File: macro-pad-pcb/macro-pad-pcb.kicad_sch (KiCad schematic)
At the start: 46 parts, among them SW1 SW_Push, SW2 RotaryEncoder, U1 PRTR5V0U2X, U2 ATmega32U4-A, Y1 Crystal_GND24_Small

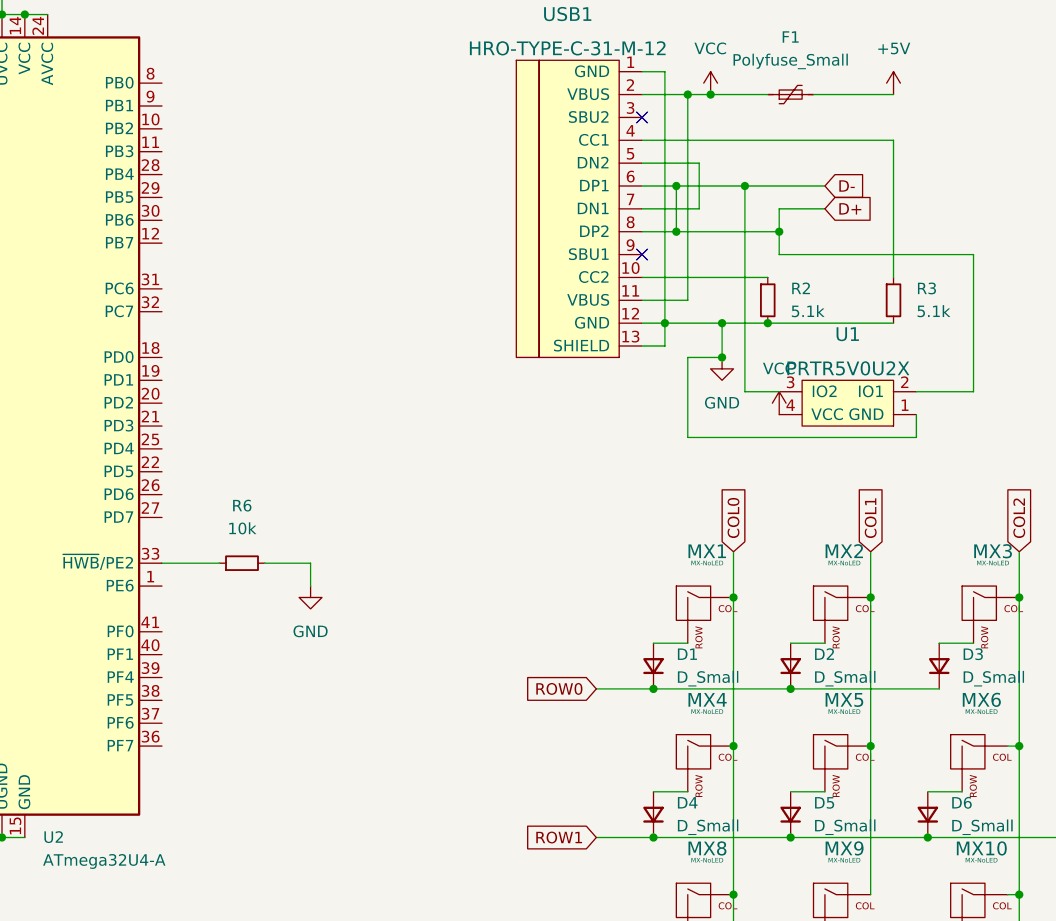
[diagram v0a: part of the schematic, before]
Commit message: Finished PCB
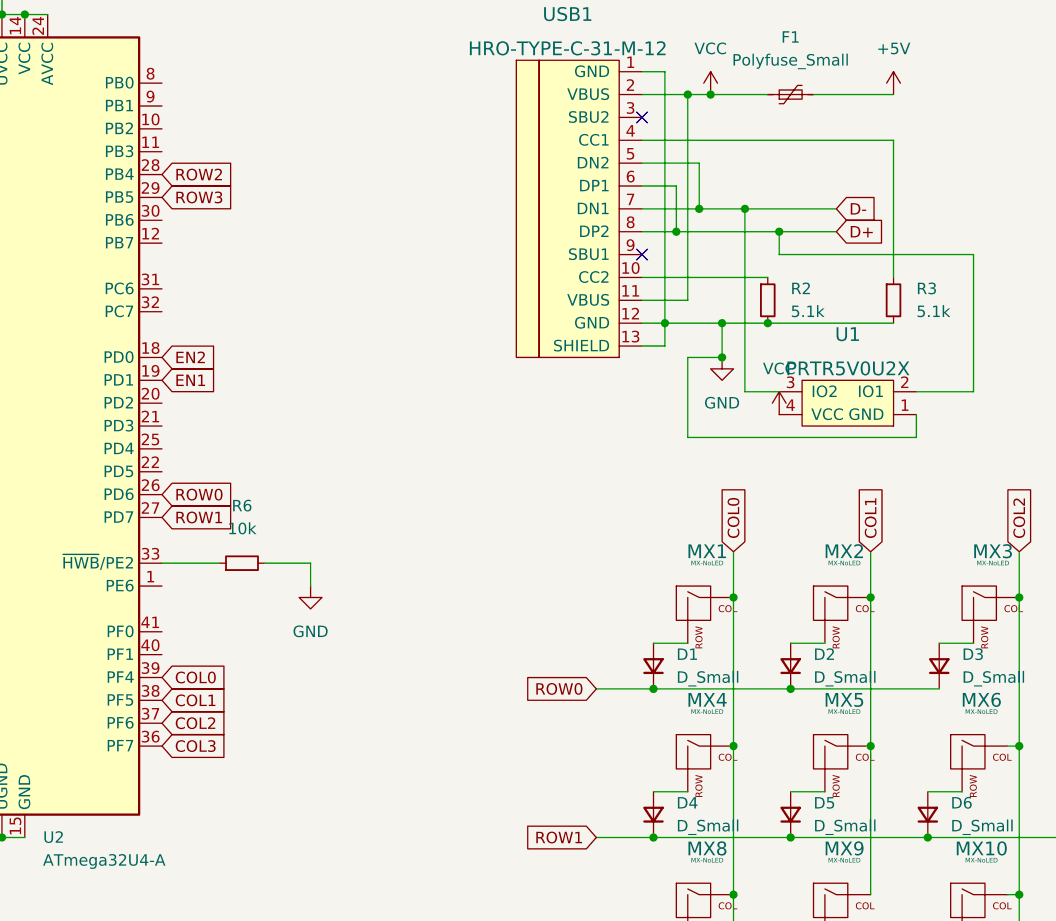
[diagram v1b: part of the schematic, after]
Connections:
- net COL0: now also U2.39 (PF4)
- net COL1: now also U2.38 (PF5)
- net COL2: now also U2.37 (PF6)
- net COL3: now also U2.36 (PF7)
- net D+: no longer R5.1, U1.3 (IO2)
- net EN1: now also U2.19 (PD1)
- net EN2: now also U2.18 (PD0)
- net ROW0: now also U2.26 (PD6)
- net ROW1: now also U2.27 (PD7)
- net ROW2: now also U2.28 (PB4)
- net ROW3: now also U2.29 (PB5)
- net D-: now reaches USB1.5 (DN2), USB1.7 (DN1)
- net D-: now also R5.1, U1.3 (IO2)
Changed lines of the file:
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@@
   (junction (at 50.8 31.75) (diameter 0) (color 0 0 0 0)
   )
-  (junction (at 133.35 50.8) (diameter 0) (color 0 0 0 0)
-  )
   (junction (at 36.83 49.53) (diameter 0) (color 0 0 0 0)
   )
+  (junction (at 144.78 55.88) (diameter 0) (color 0 0 0 0)
+  )
   (junction (at 186.69 113.03) (diameter 0) (color 0 0 0 0)
   )
@@
   (junction (at 137.16 40.64) (diameter 0) (color 0 0 0 0)
   )
-  (junction (at 144.78 55.88) (diameter 0) (color 0 0 0 0)
-  )
   (junction (at 130.81 106.68) (diameter 0) (color 0 0 0 0)
   )
   (junction (at 139.7 96.52) (diameter 0) (color 0 0 0 0)
   )
+  (junction (at 135.89 53.34) (diameter 0) (color 0 0 0 0)
+  )
   (junction (at 139.7 129.54) (diameter 0) (color 0 0 0 0)
   )
+  (junction (at 140.97 53.34) (diameter 0) (color 0 0 0 0)
+  )
   (junction (at 161.29 123.19) (diameter 0) (color 0 0 0 0)
   )
@@
   )
   (junction (at 154.94 113.03) (diameter 0) (color 0 0 0 0)
-  )
-  (junction (at 140.97 50.8) (diameter 0) (color 0 0 0 0)
   )
   (junction (at 146.05 139.7) (diameter 0) (color 0 0 0 0)
@@
     (stroke (width 0) (type default) (color 0 0 0 0))
   )
-  (wire (pts (xy 144.78 53.34) (xy 149.86 53.34))
-    (stroke (width 0) (type default) (color 0 0 0 0))
-  )
   (wire (pts (xy 15.24 95.25) (xy 25.4 95.25))
     (stroke (width 0) (type default) (color 0 0 0 0))
@@
     (stroke (width 0) (type default) (color 0 0 0 0))
   )
-  (wire (pts (xy 144.78 55.88) (xy 144.78 53.34))
-    (stroke (width 0) (type default) (color 0 0 0 0))
-  )
   (wire (pts (xy 38.1 64.77) (xy 45.72 64.77))
     (stroke (width 0) (type default) (color 0 0 0 0))
@@
     (stroke (width 0) (type default) (color 0 0 0 0))
   )
-  (wire (pts (xy 140.97 73.66) (xy 140.97 50.8))
-    (stroke (width 0) (type default) (color 0 0 0 0))
-  )
   (wire (pts (xy 124.46 106.68) (xy 130.81 106.68))
     (stroke (width 0) (type default) (color 0 0 0 0))
@@
     (stroke (width 0) (type default) (color 0 0 0 0))
   )
+  (wire (pts (xy 144.78 55.88) (xy 151.13 55.88))
+    (stroke (width 0) (type default) (color 0 0 0 0))
+  )
   (wire (pts (xy 129.54 50.8) (xy 133.35 50.8))
     (stroke (width 0) (type default) (color 0 0 0 0))
@@
     (stroke (width 0) (type default) (color 0 0 0 0))
   )
-  (wire (pts (xy 133.35 50.8) (xy 140.97 50.8))
+  (wire (pts (xy 135.89 53.34) (xy 140.97 53.34))
+    (stroke (width 0) (type default) (color 0 0 0 0))
+  )
+  (wire (pts (xy 140.97 53.34) (xy 140.97 73.66))
     (stroke (width 0) (type default) (color 0 0 0 0))
   )
@@
     (stroke (width 0) (type default) (color 0 0 0 0))
   )
-  (wire (pts (xy 140.97 50.8) (xy 149.86 50.8))
-    (stroke (width 0) (type default) (color 0 0 0 0))
-  )
   (wire (pts (xy 130.81 134.62) (xy 134.62 134.62))
     (stroke (width 0) (type default) (color 0 0 0 0))
@@
   )
   (wire (pts (xy 196.85 97.79) (xy 209.55 97.79))
+    (stroke (width 0) (type default) (color 0 0 0 0))
+  )
+  (wire (pts (xy 140.97 53.34) (xy 151.13 53.34))
     (stroke (width 0) (type default) (color 0 0 0 0))
   )
@@
     (effects (font (size 1.27 1.27)) (justify left bottom))
   )
-  (global_label "D-" (shape input) (at 149.86 50.8 0) (fields_autoplaced)
-    (effects (font (size 1.27 1.27)) (justify left))
-    (property "Intersheet References" "${INTERSHEET_REFS}" (id 0) (at 155.1155 50.8794 0)
+  (global_label "ROW2" (shape input) (at 76.2 49.53 0) (fields_autoplaced)
+    (effects (font (size 1.27 1.27)) (justify left))
+    (property "Intersheet References" "${INTERSHEET_REFS}" (id 0) (at 83.8745 49.6094 0)
+      (effects (font (size 1.27 1.27)) (justify left) hide)
+    )
+  )
+  (global_label "D-" (shape input) (at 151.13 53.34 0) (fields_autoplaced)
+    (effects (font (size 1.27 1.27)) (justify left))
+    (property "Intersheet References" "${INTERSHEET_REFS}" (id 0) (at 156.3855 53.4194 0)
+      (effects (font (size 1.27 1.27)) (justify left) hide)
+    )
+  )
+  (global_label "EN2" (shape input) (at 76.2 69.85 0) (fields_autoplaced)
+    (effects (font (size 1.27 1.27)) (justify left))
+    (property "Intersheet References" "${INTERSHEET_REFS}" (id 0) (at 82.3021 69.9294 0)
       (effects (font (size 1.27 1.27)) (justify left) hide)
     )
@@
     )
   )
-  (global_label "D+" (shape input) (at 149.86 53.34 0) (fields_autoplaced)
-    (effects (font (size 1.27 1.27)) (justify left))
-    (property "Intersheet References" "${INTERSHEET_REFS}" (id 0) (at 155.1155 53.4194 0)
+  (global_label "D+" (shape input) (at 151.13 55.88 0) (fields_autoplaced)
+    (effects (font (size 1.27 1.27)) (justify left))
+    (property "Intersheet References" "${INTERSHEET_REFS}" (id 0) (at 156.3855 55.9594 0)
+      (effects (font (size 1.27 1.27)) (justify left) hide)
+    )
+  )
+  (global_label "COL0" (shape input) (at 76.2 105.41 0) (fields_autoplaced)
+    (effects (font (size 1.27 1.27)) (justify left))
+    (property "Intersheet References" "${INTERSHEET_REFS}" (id 0) (at 83.4512 105.3306 0)
+      (effects (font (size 1.27 1.27)) (justify left) hide)
+    )
+  )
+  (global_label "ROW1" (shape input) (at 76.2 87.63 0) (fields_autoplaced)
+    (effects (font (size 1.27 1.27)) (justify left))
+    (property "Intersheet References" "${INTERSHEET_REFS}" (id 0) (at 83.8745 87.7094 0)
       (effects (font (size 1.27 1.27)) (justify left) hide)
     )
@@
     )
   )
+  (global_label "COL2" (shape input) (at 76.2 110.49 0) (fields_autoplaced)
+    (effects (font (size 1.27 1.27)) (justify left))
+    (property "Intersheet References" "${INTERSHEET_REFS}" (id 0) (at 83.4512 110.4106 0)
+      (effects (font (size 1.27 1.27)) (justify left) hide)
+    )
+  )
+  (global_label "EN1" (shape input) (at 76.2 72.39 0) (fields_autoplaced)
+    (effects (font (size 1.27 1.27)) (justify left))
+    (property "Intersheet References" "${INTERSHEET_REFS}" (id 0) (at 82.3021 72.4694 0)
+      (effects (font (size 1.27 1.27)) (justify left) hide)
+    )
+  )
+  (global_label "ROW3" (shape input) (at 76.2 52.07 0) (fields_autoplaced)
+    (effects (font (size 1.27 1.27)) (justify left))
+    (property "Intersheet References" "${INTERSHEET_REFS}" (id 0) (at 83.8745 52.1494 0)
+      (effects (font (size 1.27 1.27)) (justify left) hide)
+    )
+  )
   (global_label "EN2" (shape input) (at 209.55 95.25 180) (fields_autoplaced)
     (effects (font (size 1.27 1.27)) (justify right))
@@
     )
   )
+  (global_label "COL1" (shape input) (at 76.2 107.95 0) (fields_autoplaced)
+    (effects (font (size 1.27 1.27)) (justify left))
+    (property "Intersheet References" "${INTERSHEET_REFS}" (id 0) (at 83.4512 107.8706 0)
+      (effects (font (size 1.27 1.27)) (justify left) hide)
+    )
+  )
   (global_label "COL2" (shape input) (at 171.45 91.44 90) (fields_autoplaced)
     (effects (font (size 1.27 1.27)) (justify left))
@@
     )
   )
+  (global_label "ROW0" (shape input) (at 76.2 85.09 0) (fields_autoplaced)
+    (effects (font (size 1.27 1.27)) (justify left))
+    (property "Intersheet References" "${INTERSHEET_REFS}" (id 0) (at 83.8745 85.1694 0)
+      (effects (font (size 1.27 1.27)) (justify left) hide)
+    )
+  )
   (global_label "D-" (shape input) (at 26.67 67.31 180) (fields_autoplaced)
     (effects (font (size 1.27 1.27)) (justify right))
@@
     )
   )
+  (global_label "COL3" (shape input) (at 76.2 113.03 0) (fields_autoplaced)
+    (effects (font (size 1.27 1.27)) (justify left))
+    (property "Intersheet References" "${INTERSHEET_REFS}" (id 0) (at 83.4512 112.9506 0)
+      (effects (font (size 1.27 1.27)) (justify left) hide)
+    )
+  )
